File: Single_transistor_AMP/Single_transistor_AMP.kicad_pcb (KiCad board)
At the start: 2 copper layers, 57.2 x 41.9 mm, 11 parts, among them J1 Conn_01x02, J2 Conn_01x02, J3 Screw_Terminal_01x02, Q1 2N2219

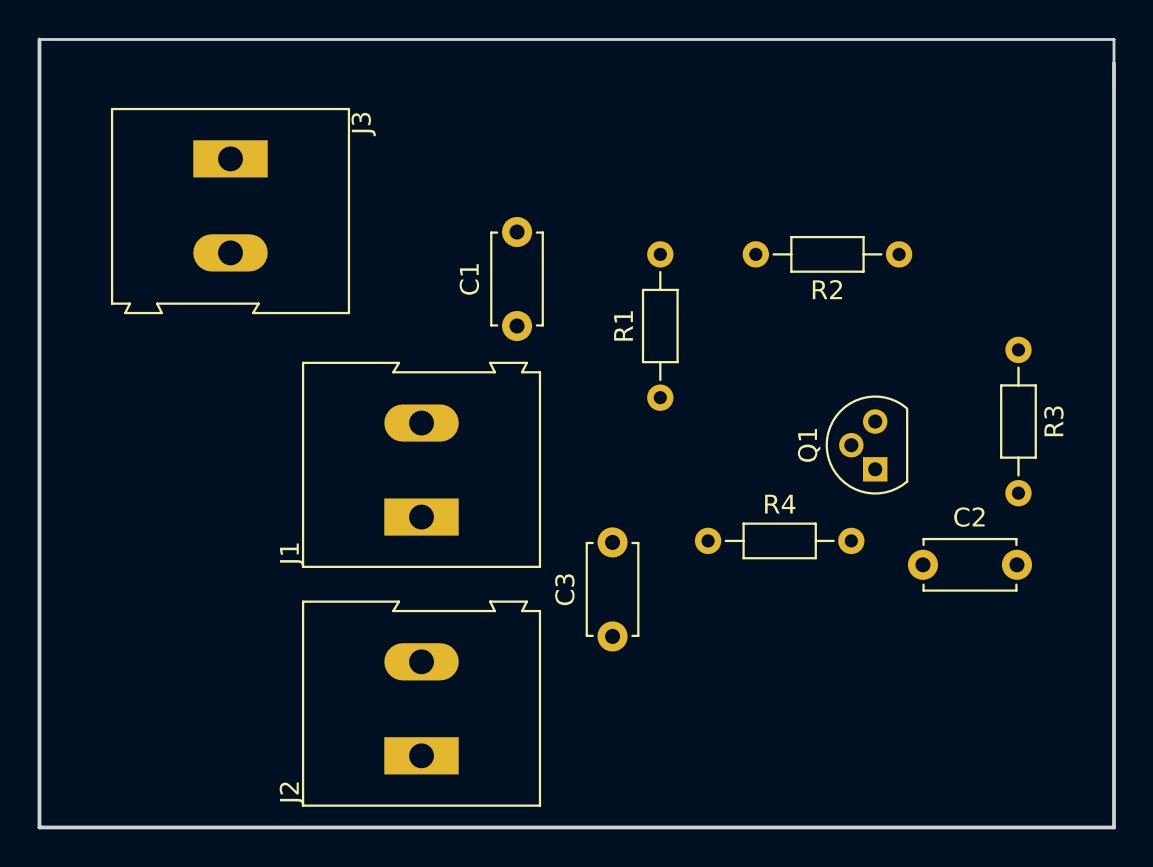
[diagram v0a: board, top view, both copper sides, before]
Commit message: first commiRtF
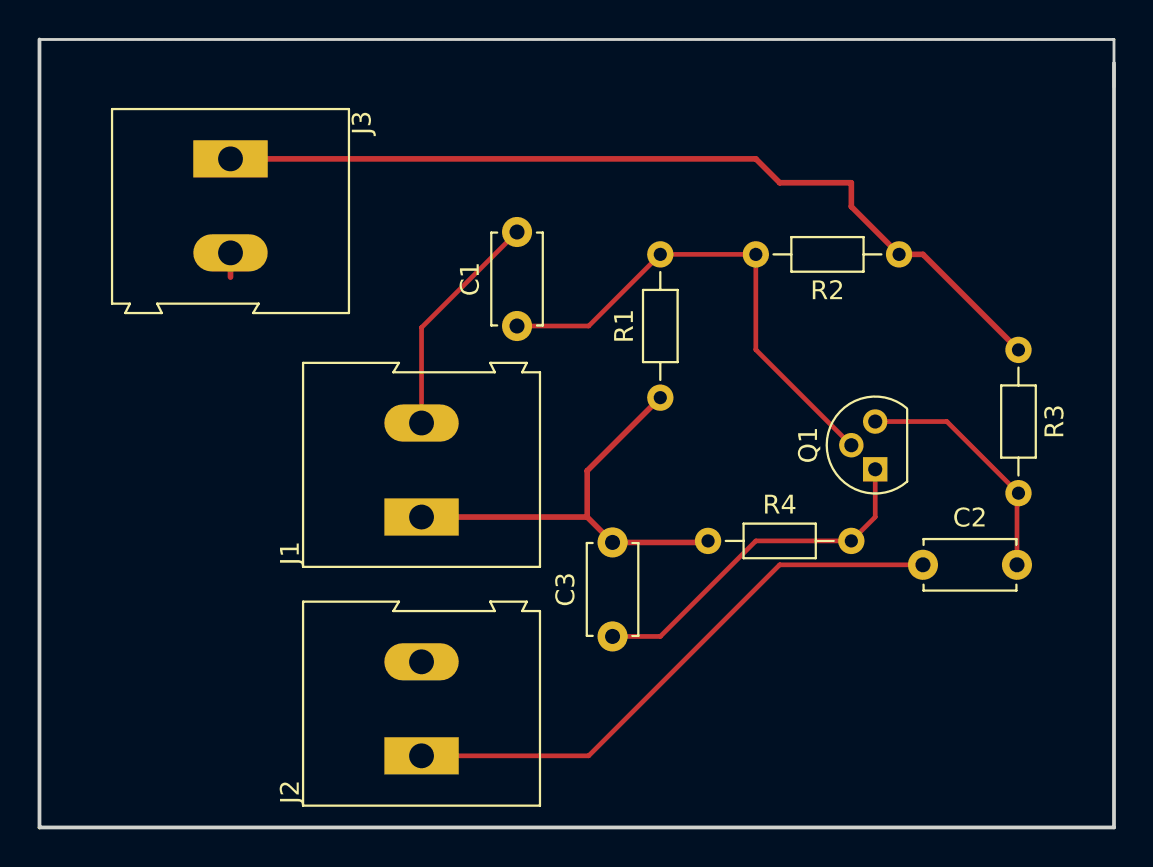
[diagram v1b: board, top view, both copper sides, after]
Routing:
- net VCC: track 0.00 -> 46.9 mm
- net Net-(C2-Pad1): track 0.00 -> 30.9 mm
- net Net-(C1-Pad1): track 0.00 -> 26.5 mm
- net GND: track 0.00 -> 26.1 mm
- net Net-(C3-Pad1): track 0.00 -> 19.1 mm
- net Net-(C2-Pad2): track 0.00 -> 13.0 mm
- net Net-(C1-Pad2): track 0.00 -> 12.3 mm
- added copper zone on B.Cu, net GND
- added copper zone on F.Cu, net GND

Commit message: first commiRtdfF
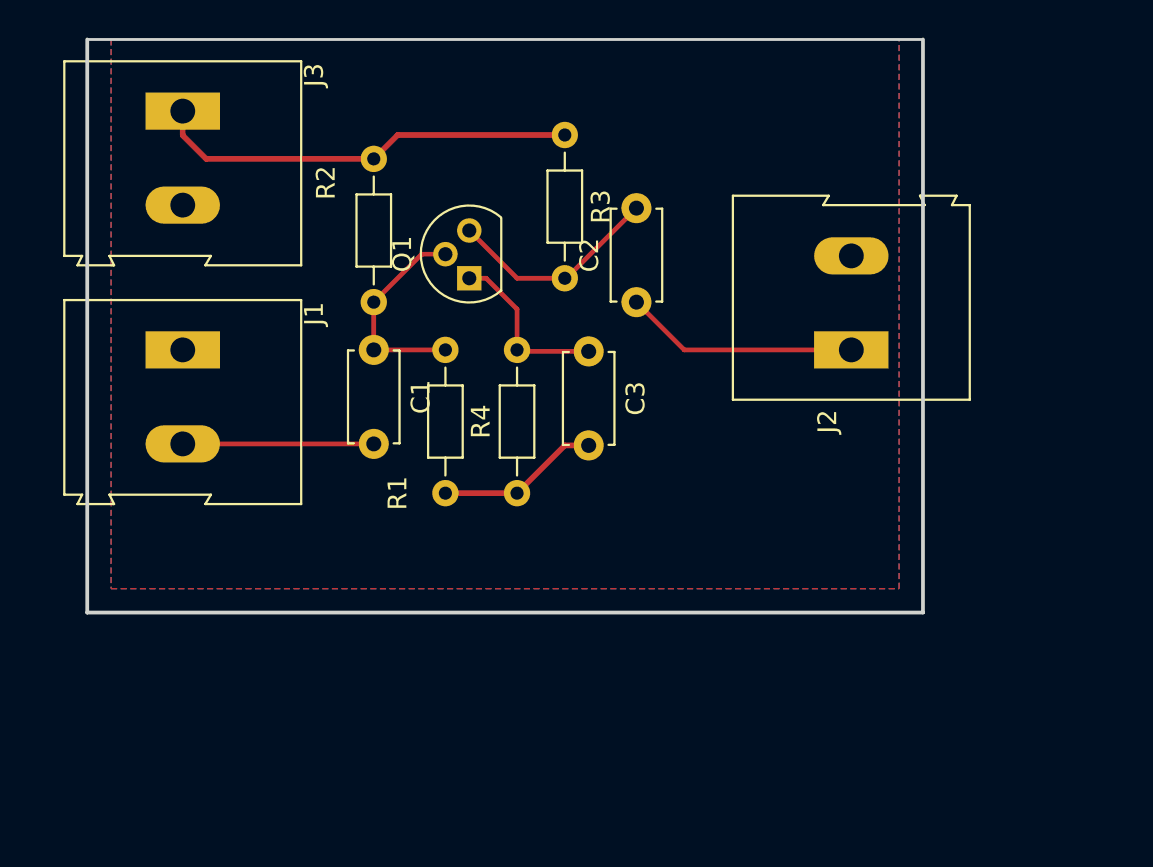
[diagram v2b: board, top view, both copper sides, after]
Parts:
- moved J2 31.4 mm to (134.6, 55.9)
- moved R2 28.4 mm to (109.2, 45.7), turned to 270 degrees
- moved R3 26.7 mm to (119.4, 44.5)
- moved Q1 23.9 mm to (114.3, 52.1)
- moved C2 20.7 mm to (123.2, 53.3), turned to 90 degrees
- moved J1 15.5 mm to (99.1, 55.9), turned to 270 degrees
- moved C3 15.2 mm to (120.7, 56.0), turned to 270 degrees
- moved R1 12.5 mm to (113.0, 63.5)
- moved R4 10.5 mm to (116.8, 63.5), turned to 90 degrees
- moved C1 7.73 mm to (109.2, 55.9), turned to 270 degrees
- moved J3 3.59 mm to (99.1, 43.2)
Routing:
- net VCC: track 46.9 -> 22.7 mm
- net Net-(C2-Pad1): track 30.9 -> 12.5 mm
- net GND: track 26.1 -> 8.67 mm
- net Net-(C1-Pad1): track 26.5 -> 11.2 mm
- net Net-(C3-Pad1): track 19.1 -> 9.23 mm
- net Net-(C1-Pad2): track 12.3 -> 10.2 mm
- net Net-(C2-Pad2): track 13.0 -> 11.5 mm
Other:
- board size 57.2 x 41.9 mm -> 44.5 x 30.5 mm

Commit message: first commiRtdfFd
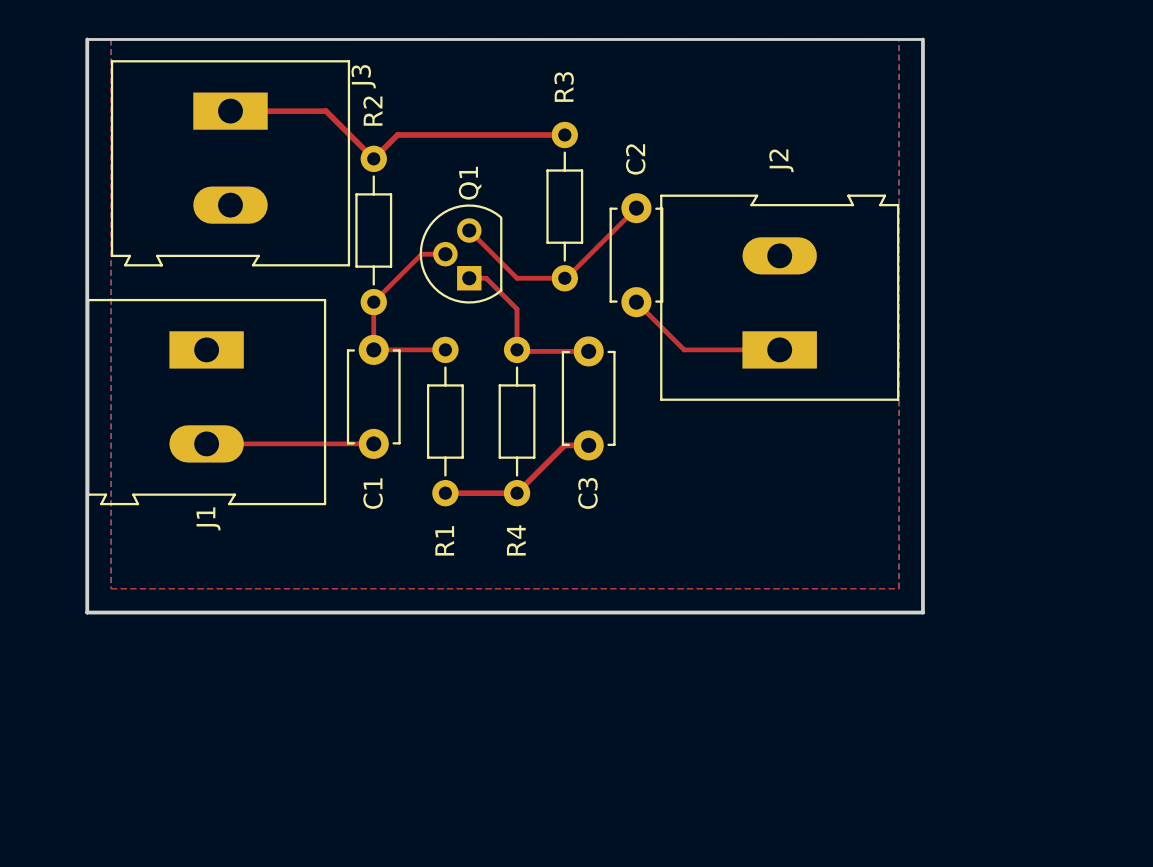
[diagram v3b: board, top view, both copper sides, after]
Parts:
- moved J2 3.81 mm to (130.8, 55.9)
- moved J3 2.54 mm to (101.6, 43.2)
- moved J1 1.27 mm to (100.3, 55.9)
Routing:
- net Net-(C2-Pad1): track 12.5 -> 8.67 mm
- net VCC: track 22.7 -> 19.4 mm
- net Net-(C1-Pad2): track 10.2 -> 8.89 mm
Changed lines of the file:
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@@
     (thickness 1.6)
     (drawings 4)
-    (tracks 24)
+    (tracks 23)
     (zones 0)
     (modules 11)
@@
     (visible_elements 7FFFF7FF)
     (pcbplotparams
-      (layerselection 0x010f0_ffffffff)
+      (layerselection 0x010e0_ffffffff)
       (usegerberextensions false)
       (usegerberattributes false)
@@
   )
   (module TerminalBlock:TerminalBlock_Altech_AK300-2_P5.00mm (layer F.Cu)
-    (at 99.06 55.88 270)
+    (at 100.33 55.88 270)
     (descr "Altech AK300 terminal block, pitch 5.0mm, 45 degree angled, see http://www.mouser.com/ds/2/16/PCBMETRC-24178.pdf")
     (tags "Altech AK300 terminal block pitch 5.0mm")
-    (fp_text reference J1 (at -1.92 -6.99 270) (layer F.SilkS)
+    (fp_text reference J1 (at 8.89 0 270) (layer F.SilkS)
       (effects (font (size 1 1) (thickness 0.15)))
     )
@@
     (descr "C, Disc series, Radial, pin pitch=5.00mm, , diameter*width=4.7*2.5mm^2, Capacitor, http://www.vishay.com/docs/45233/krseries.pdf")
     (tags "C Disc series Radial pin pitch 5.00mm  diameter 4.7mm width 2.5mm Capacitor")
-    (fp_text reference C1 (at 2.5 -2.5 270) (layer F.SilkS)
+    (fp_text reference C1 (at 7.62 0 270) (layer F.SilkS)
       (effects (font (size 1 1) (thickness 0.15)))
     )
@@
     (descr "C, Disc series, Radial, pin pitch=5.00mm, , diameter*width=4.7*2.5mm^2, Capacitor, http://www.vishay.com/docs/45233/krseries.pdf")
     (tags "C Disc series Radial pin pitch 5.00mm  diameter 4.7mm width 2.5mm Capacitor")
-    (fp_text reference C2 (at 2.5 -2.5 90) (layer F.SilkS)
+    (fp_text reference C2 (at 7.62 0 90) (layer F.SilkS)
       (effects (font (size 1 1) (thickness 0.15)))
     )
@@
     (descr "C, Disc series, Radial, pin pitch=5.00mm, , diameter*width=4.7*2.5mm^2, Capacitor, http://www.vishay.com/docs/45233/krseries.pdf")
     (tags "C Disc series Radial pin pitch 5.00mm  diameter 4.7mm width 2.5mm Capacitor")
-    (fp_text reference C3 (at 2.5 -2.5 270) (layer F.SilkS)
+    (fp_text reference C3 (at 7.54 0 270) (layer F.SilkS)
       (effects (font (size 1 1) (thickness 0.15)))
     )
@@
   )
   (module TerminalBlock:TerminalBlock_Altech_AK300-2_P5.00mm (layer F.Cu)
-    (at 134.62 55.88 90)
+    (at 130.81 55.88 90)
     (descr "Altech AK300 terminal block, pitch 5.0mm, 45 degree angled, see http://www.mouser.com/ds/2/16/PCBMETRC-24178.pdf")
     (tags "Altech AK300 terminal block pitch 5.0mm")
-    (fp_text reference J2 (at -3.81 -1.27 90) (layer F.SilkS)
+    (fp_text reference J2 (at 10.16 0 90) (layer F.SilkS)
       (effects (font (size 1 1) (thickness 0.15)))
     )
@@
     (descr "TO-92L leads in-line (large body variant of TO-92), also known as TO-226, wide, drill 0.75mm (see https://www.diodes.com/assets/Package-Files/TO92L.pdf and http://www.ti.com/lit/an/snoa059/snoa059.pdf)")
     (tags "TO-92L Molded Narrow transistor")
-    (fp_text reference Q1 (at 1.29 -3.56 90) (layer F.SilkS)
+    (fp_text reference Q1 (at 5.08 0 90) (layer F.SilkS)
       (effects (font (size 1 1) (thickness 0.15)))
     )
@@
     (descr "Resistor, Axial_DIN0204 series, Axial, Horizontal, pin pitch=7.62mm, 0.167W, length*diameter=3.6*1.6mm^2, http://cdn-reichelt.de/documents/datenblatt/B400/1_4W%23YAG.pdf")
     (tags "Resistor Axial_DIN0204 series Axial Horizontal pin pitch 7.62mm 0.167W length 3.6mm diameter 1.6mm")
-    (fp_text reference R1 (at 0 -2.54 90) (layer F.SilkS)
+    (fp_text reference R1 (at -2.54 0 90) (layer F.SilkS)
       (effects (font (size 1 1) (thickness 0.15)))
     )
@@
     (descr "Resistor, Axial_DIN0204 series, Axial, Horizontal, pin pitch=7.62mm, 0.167W, length*diameter=3.6*1.6mm^2, http://cdn-reichelt.de/documents/datenblatt/B400/1_4W%23YAG.pdf")
     (tags "Resistor Axial_DIN0204 series Axial Horizontal pin pitch 7.62mm 0.167W length 3.6mm diameter 1.6mm")
-    (fp_text reference R2 (at 1.27 2.54 270) (layer F.SilkS)
+    (fp_text reference R2 (at -2.54 0 270) (layer F.SilkS)
       (effects (font (size 1 1) (thickness 0.15)))
     )
@@
     (descr "Resistor, Axial_DIN0204 series, Axial, Horizontal, pin pitch=7.62mm, 0.167W, length*diameter=3.6*1.6mm^2, http://cdn-reichelt.de/documents/datenblatt/B400/1_4W%23YAG.pdf")
     (tags "Resistor Axial_DIN0204 series Axial Horizontal pin pitch 7.62mm 0.167W length 3.6mm diameter 1.6mm")
-    (fp_text reference R3 (at 3.81 -1.92 270) (layer F.SilkS)
+    (fp_text reference R3 (at -2.54 0 270) (layer F.SilkS)
       (effects (font (size 1 1) (thickness 0.15)))
     )
@@
     (descr "Resistor, Axial_DIN0204 series, Axial, Horizontal, pin pitch=7.62mm, 0.167W, length*diameter=3.6*1.6mm^2, http://cdn-reichelt.de/documents/datenblatt/B400/1_4W%23YAG.pdf")
     (tags "Resistor Axial_DIN0204 series Axial Horizontal pin pitch 7.62mm 0.167W length 3.6mm diameter 1.6mm")
-    (fp_text reference R4 (at 3.81 -1.92 90) (layer F.SilkS)
+    (fp_text reference R4 (at -2.54 0 90) (layer F.SilkS)
       (effects (font (size 1 1) (thickness 0.15)))
     )
@@
   )
   (module TerminalBlock:TerminalBlock_Altech_AK300-2_P5.00mm (layer F.Cu)
-    (at 99.06 43.18 270)
+    (at 101.6 43.18 270)
     (descr "Altech AK300 terminal block, pitch 5.0mm, 45 degree angled, see http://www.mouser.com/ds/2/16/PCBMETRC-24178.pdf")
     (tags "Altech AK300 terminal block pitch 5.0mm")
@@
   (segment (start 111.77 50.79) (end 109.22 53.34) (width 0.25) (layer F.Cu) (net 1))
   (segment (start 113.03 50.79) (end 111.77 50.79) (width 0.25) (layer F.Cu) (net 1))
-  (segment (start 109.22 60.88) (end 99.06 60.88) (width 0.25) (layer F.Cu) (net 2))
+  (segment (start 100.33 60.88) (end 109.22 60.88) (width 0.25) (layer F.Cu) (net 2))
   (segment (start 125.73 55.88) (end 123.19 53.34) (width 0.25) (layer F.Cu) (net 3))
-  (segment (start 134.62 55.88) (end 125.73 55.88) (width 0.25) (layer F.Cu) (net 3))
+  (segment (start 130.81 55.88) (end 125.73 55.88) (width 0.25) (layer F.Cu) (net 3))
   (segment (start 116.84 52.07) (end 114.3 49.53) (width 0.25) (layer F.Cu) (net 4))
   (segment (start 119.38 52.07) (end 116.84 52.07) (width 0.25) (layer F.Cu) (net 4))
@@
   (segment (start 116.92 55.96) (end 116.84 55.88) (width 0.25) (layer F.Cu) (net 6))
   (segment (start 120.65 55.96) (end 116.92 55.96) (width 0.25) (layer F.Cu) (net 6))
-  (segment (start 99.06 44.47) (end 99.06 43.18) (width 0.3) (layer F.Cu) (net 7))
-  (segment (start 100.31 45.72) (end 99.06 44.47) (width 0.3) (layer F.Cu) (net 7))
-  (segment (start 109.22 45.72) (end 100.31 45.72) (width 0.3) (layer F.Cu) (net 7))
   (segment (start 110.49 44.45) (end 109.22 45.72) (width 0.3) (layer F.Cu) (net 7))
   (segment (start 119.38 44.45) (end 110.49 44.45) (width 0.3) (layer F.Cu) (net 7))
+  (segment (start 106.68 43.18) (end 109.22 45.72) (width 0.3) (layer F.Cu) (net 7))
+  (segment (start 101.6 43.18) (end 106.68 43.18) (width 0.3) (layer F.Cu) (net 7))
   (zone (net 5) (net_name GND) (layer F.Cu) (hatch edge 0.508)
     (connect_pads (clearance 0.508))
